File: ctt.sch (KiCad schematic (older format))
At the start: 7 parts, among them CN1 CONN_3, CN2 CONN_3, J1 RELAY

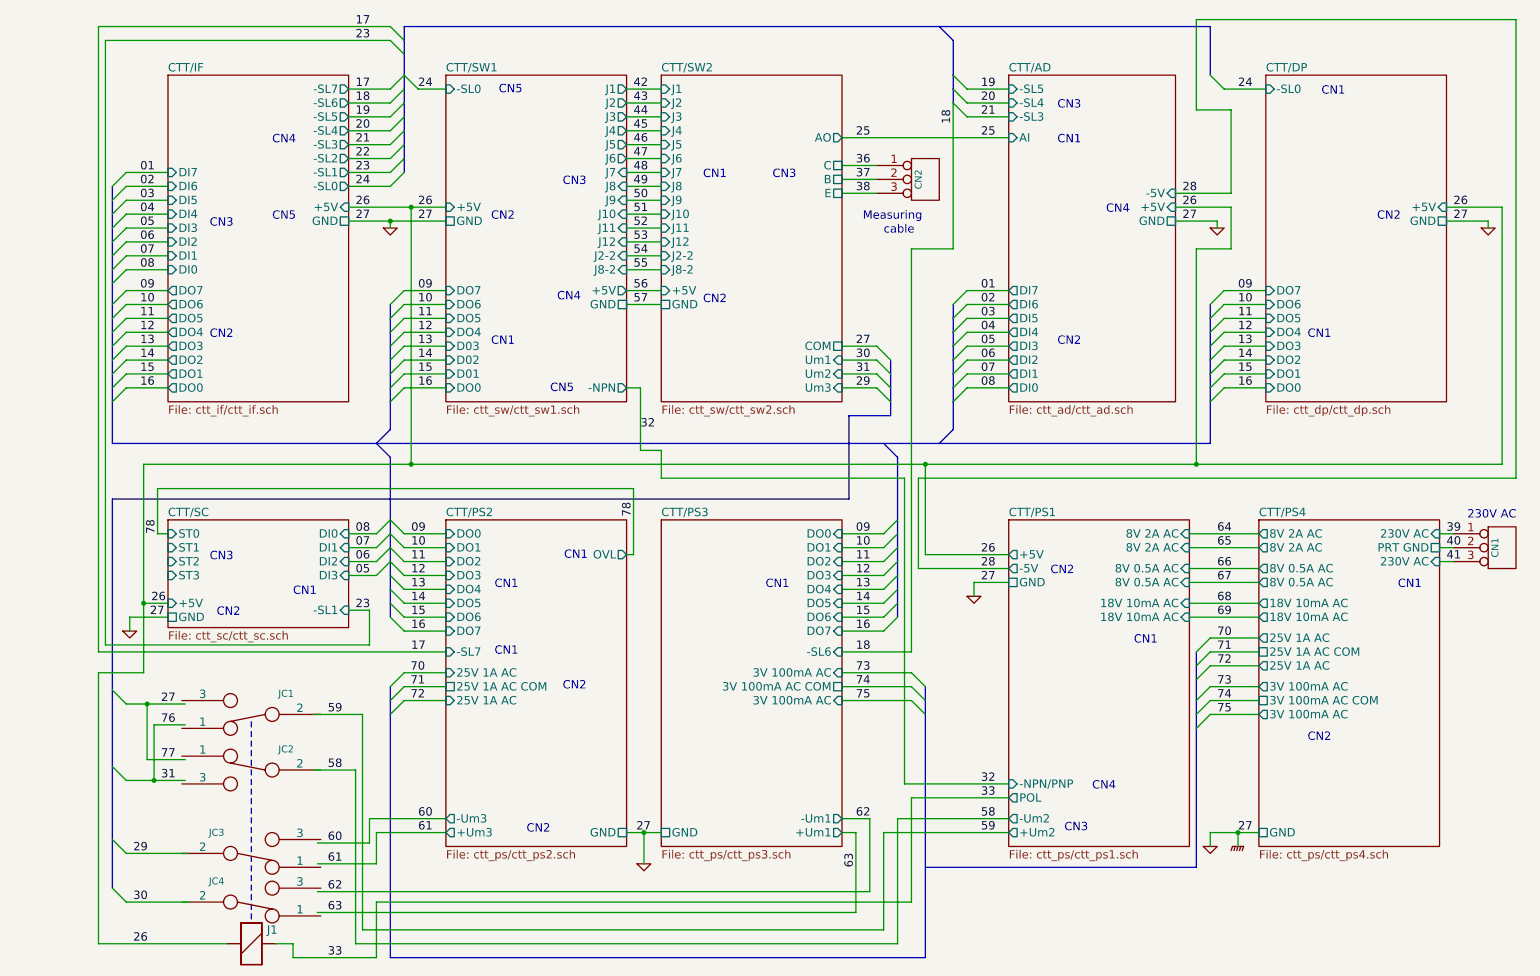
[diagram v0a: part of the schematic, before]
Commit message: 08.07-i állapot.
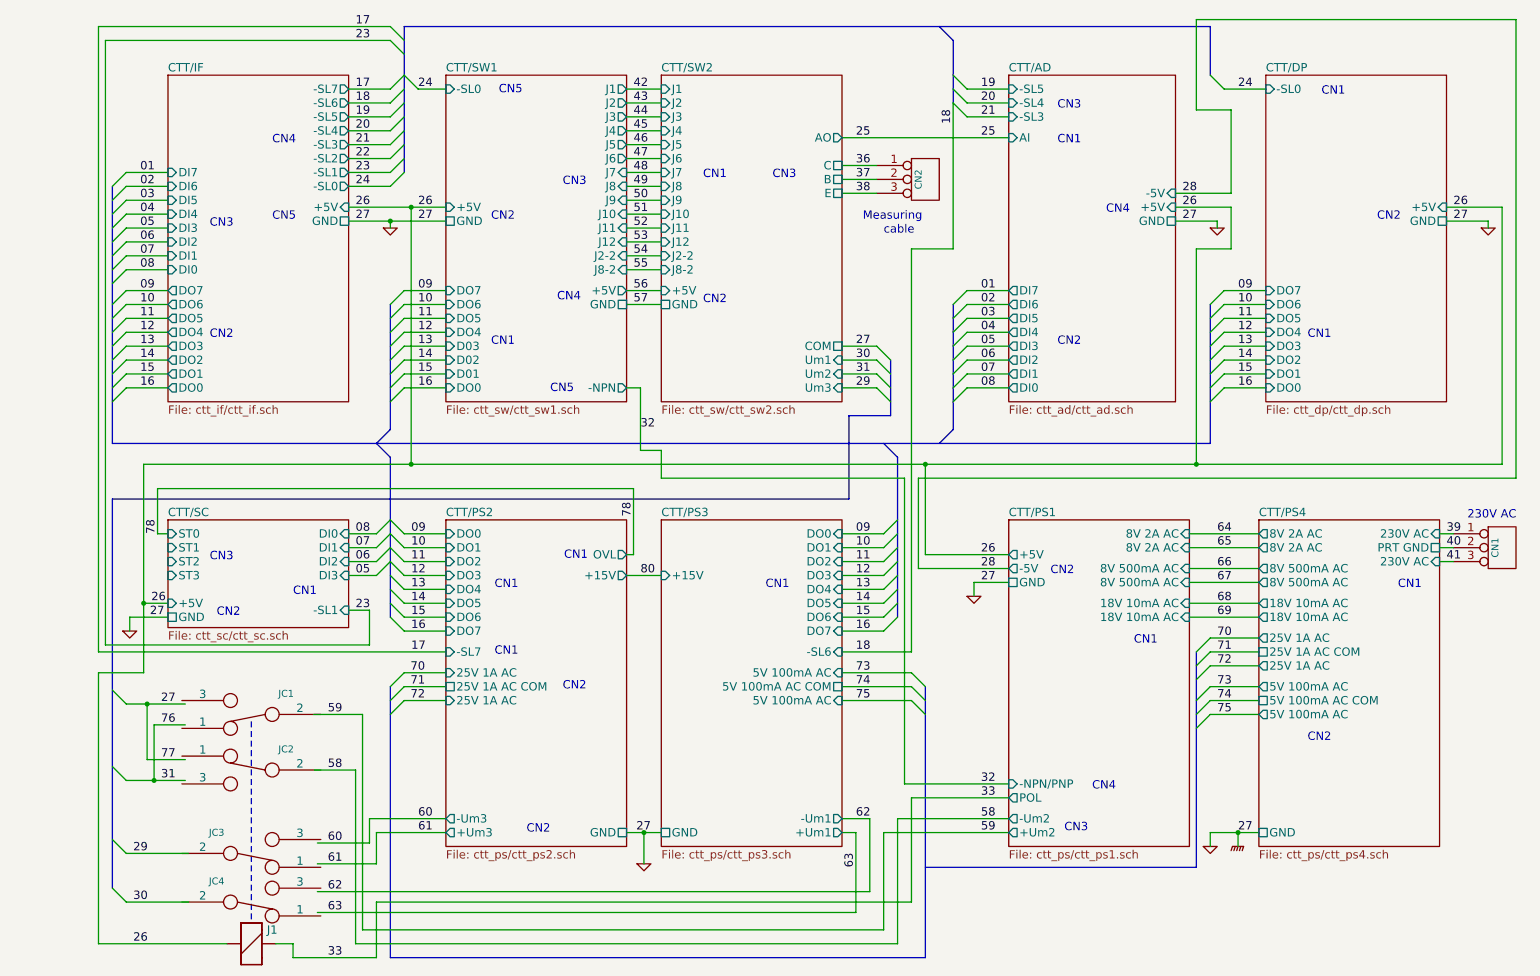
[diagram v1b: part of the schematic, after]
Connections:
- net labels added: 80
- wire segments 230 -> 220
